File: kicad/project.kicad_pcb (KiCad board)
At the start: 2 copper layers, 59 x 59 mm, 33 parts, among them J1 Conn_01x05, J2 Conn_01x01, SW1 SW_DPDT_x2, U1 STM32L031F4Px

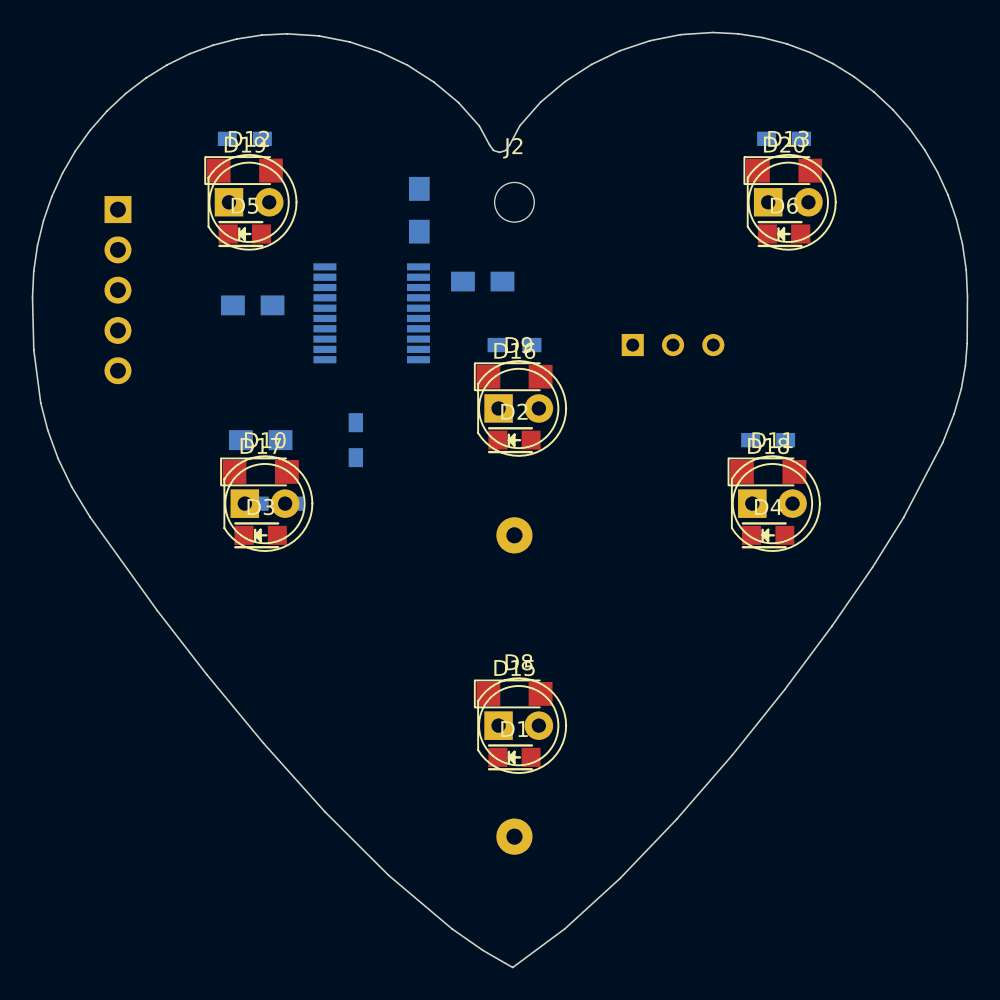
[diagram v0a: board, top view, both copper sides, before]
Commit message: Routing
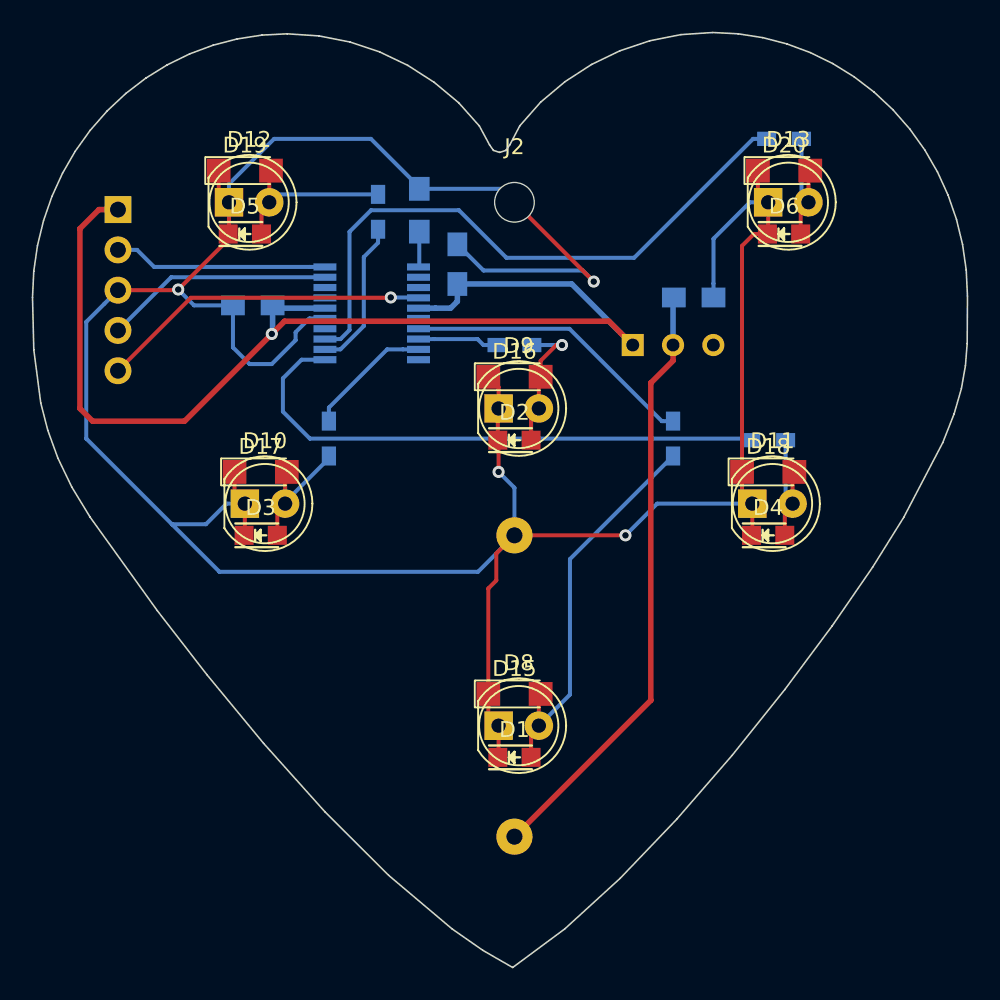
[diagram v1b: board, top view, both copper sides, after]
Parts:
- J1: footprint Pin_Header_Straight_1x05_Pitch2.54mm -> Pin_Headers:Pin_Header_Straight_1x05_Pitch2.54mm
- moved C1 28.7 mm to (141.3, 102.0), turned to 0 degrees
- moved R2 20.0 mm to (140.0, 110.9)
- moved R6 9.58 mm to (121.4, 96.6), turned to 270 degrees
- moved R4 5.26 mm to (118.3, 110.9), turned to 90 degrees
- moved C3 1.94 mm to (126.4, 99.9), turned to 270 degrees
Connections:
- net Net-(BT1-Pad1) renamed /BATT_UNSWITCHED
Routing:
- net GND: track 0.00 -> 191.3 mm, vias 0 -> 4
- net +BATT: track 0.00 -> 74.3 mm, vias 0 -> 1
- net Net-(R7-Pad2): track 0.00 -> 39.2 mm
- net /BATT_UNSWITCHED: track 0.00 -> 38.2 mm
- net Net-(R5-Pad2): track 0.00 -> 35.5 mm
- net Net-(D1-Pad2): track 0.00 -> 24.9 mm
- net NRST: track 0.00 -> 20.9 mm, vias 0 -> 1
- net Net-(R2-Pad2): track 0.00 -> 18.5 mm
- net SWDIO: track 0.00 -> 14.4 mm
- net SWCLK: track 0.00 -> 13.5 mm
- net Net-(D12-Pad2): track 0.00 -> 11.5 mm
- net Net-(R6-Pad2): track 0.00 -> 9.54 mm
- net Net-(D16-Pad2): track 0.00 -> 8.92 mm, vias 0 -> 1
- net Net-(D13-Pad2): track 0.00 -> 8.43 mm
- net Net-(D11-Pad2): track 0.00 -> 8.43 mm
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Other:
- net class Wide: clearance 0.254 -> 0.22; trace_width 0.3556 -> 0.35
